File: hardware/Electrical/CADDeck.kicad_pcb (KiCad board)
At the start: 2 copper layers, 129 x 82.5 mm, 44 parts, among them J1 Conn_01x05_Socket, J4 Conn_01x04_Socket, J5 Conn_01x10_Socket, Q1 2N2222, SW1 SW_Push, SW10 SW_Push, SW2 SW_Push, SW3 SW_Push, SW4 SW_Push, SW5 SW_Push, SW6 SW_Push, SW7 SW_Push, SW8 SW_Push, SW9 SW_Push, U1 PCF8575PWE4

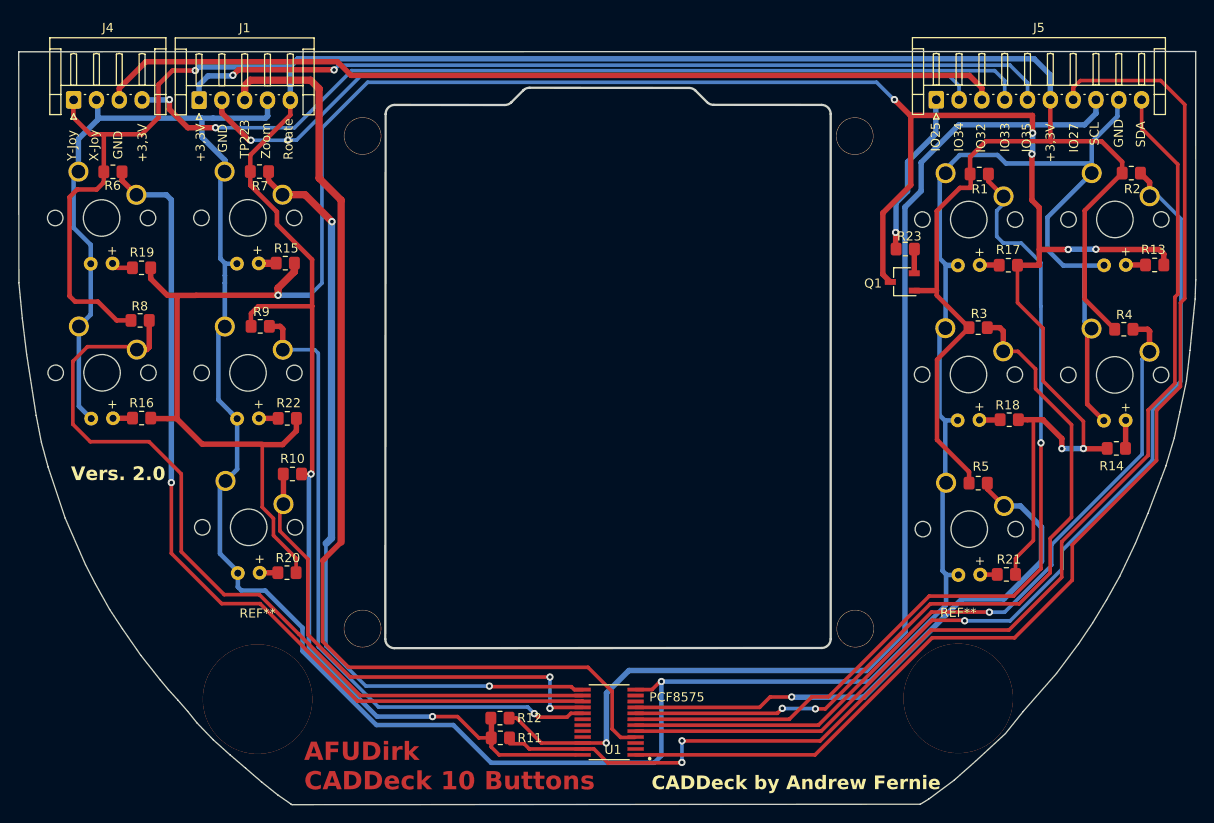
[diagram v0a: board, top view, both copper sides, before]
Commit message: Bilder aktualisiert
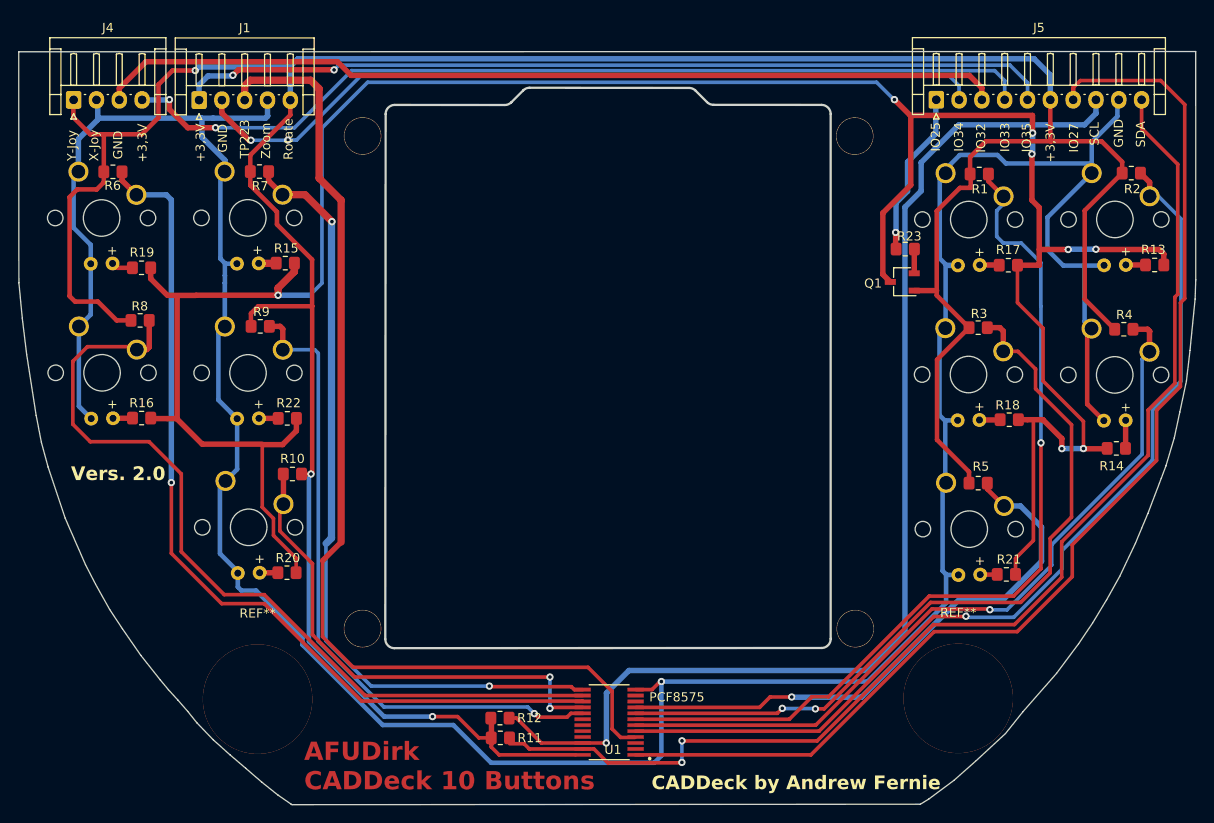
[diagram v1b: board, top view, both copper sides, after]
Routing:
- net GND: track 335.1 -> 334.0 mm
